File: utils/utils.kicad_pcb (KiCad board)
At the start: 2 copper layers, 34.8 x 69.8 mm, 22 parts, among them J6 EURORACK_CONN_16, Q1 2N3904, Q2 2N3904, Q3 2N3904, U1 TL074, U2 DG403

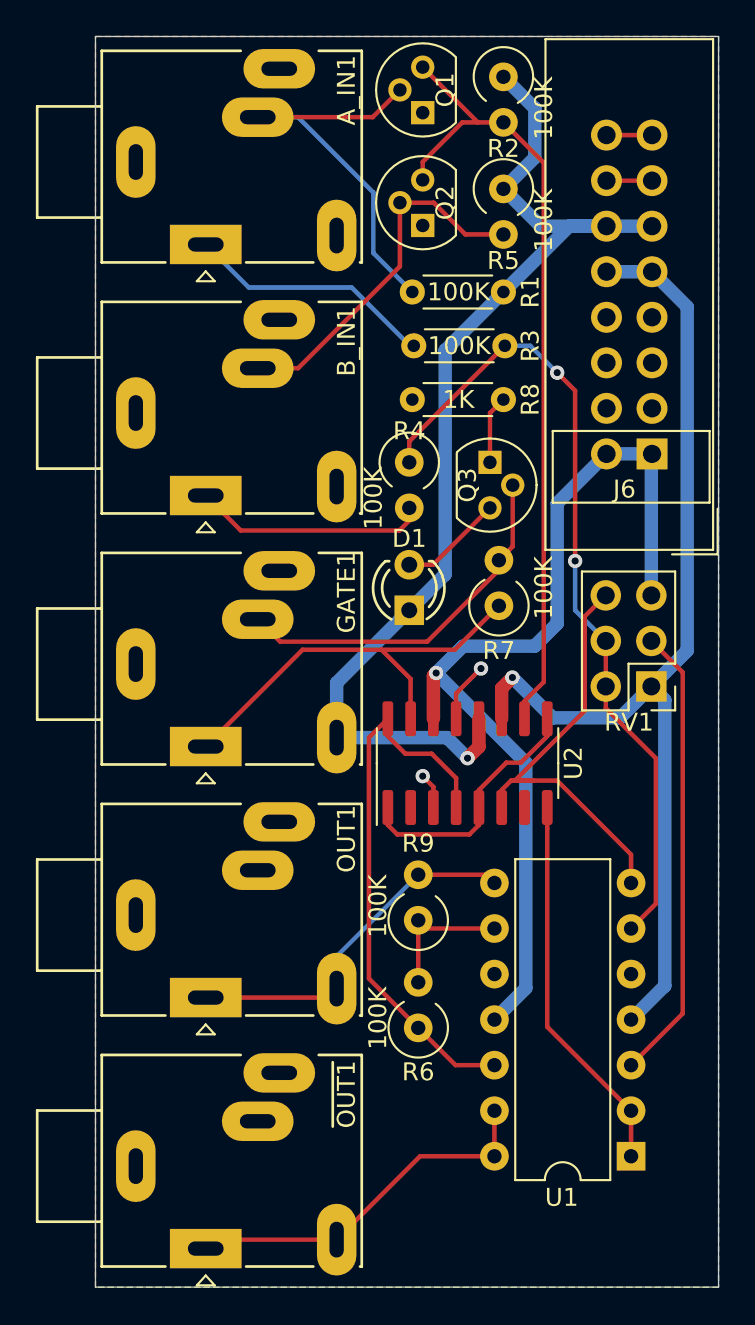
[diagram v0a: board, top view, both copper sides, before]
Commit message: cleanup
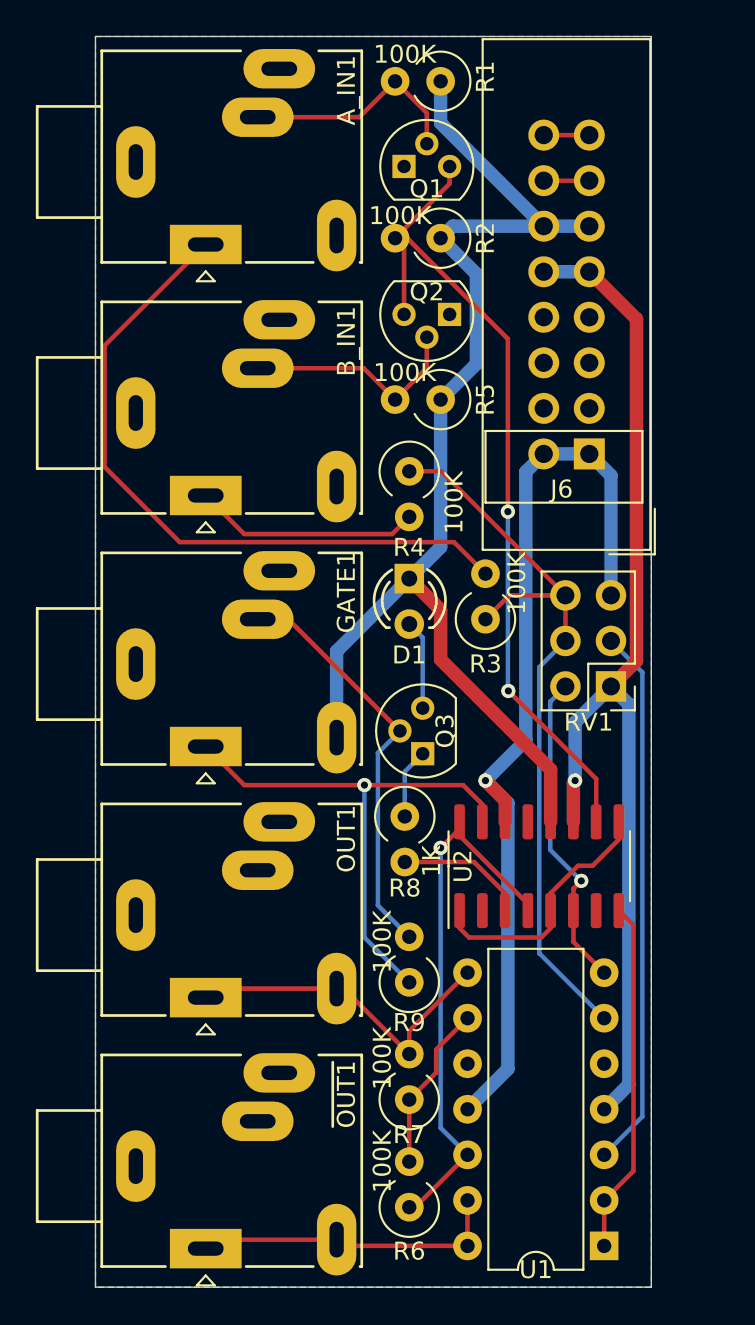
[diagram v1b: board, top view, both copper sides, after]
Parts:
- R1, R3, R8: footprint Resistor_THT:R_Axial_DIN0204_L3.6mm_D1.6mm_P5.08mm_Horizontal -> Resistor_THT:R_Axial_DIN0309_L9.0mm_D3.2mm_P2.54mm_Vertical
- moved R8 23.9 mm to (140.5, 86.5), turned to 270 degrees
- moved R7 21.6 mm to (140.8, 95.8)
- moved Q3 16.7 mm to (141.5, 83.0), turned to 90 degrees
- moved R3 15.3 mm to (145.0, 75.5), turned to 90 degrees
- moved R1 12.3 mm to (142.5, 45.5)
- moved R5 12.3 mm to (142.5, 63.2), turned to 180 degrees
- moved R6 10.0 mm to (140.8, 108.3)
- moved R9 10.0 mm to (140.8, 102.3)
- moved R2 9.66 mm to (142.5, 54.2), turned to 180 degrees
- moved U2 7.00 mm to (148.0, 89.3)
- moved U1 5.22 mm to (151.6, 110.5)
- moved Q2 5.18 mm to (143.0, 58.5), turned to 180 degrees
- moved J6 3.50 mm to (150.8, 66.3)
- moved Q1 3.18 mm to (140.5, 50.2), turned to 0 degrees
- moved RV1 2.25 mm to (152.0, 79.2)
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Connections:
- RV1 pad 4: Net-(R3-Pad1) -> Net-(RV1-Pad4)
- RV1 pad 6: Net-(RV1-Pad6) -> Net-(R3-Pad1)
- U1 pad 7: Net-(RV1-Pad6) -> Net-(RV1-Pad4)
- U2 pad 6: Net-(RV1-Pad6) -> Net-(RV1-Pad4)
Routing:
- net Net-(RV1-Pad6): track 25.6 -> 0.00 mm
- net AIN: track 13.7 -> 38.5 mm
- net Net-(RV1-Pad4): track 0.00 -> 17.9 mm, vias 0 -> 1
- net A_CONN: track 23.2 -> 12.7 mm
- net B_CONN: track 20.3 -> 12.6 mm
- net GATE: track 24.1 -> 29.8 mm, vias 0 -> 1
- net Net-(RV1-Pad2): track 25.6 -> 30.3 mm
- net ~OUT: track 21.9 -> 17.5 mm
- net Net-(R3-Pad1): track 46.1 -> 42.3 mm, vias 2 -> 0
- net +5V: track 64.3 -> 67.8 mm, vias 1 -> 0
- net GATE_CONN: track 20.7 -> 23.2 mm
- net GND: track 5.75 -> 7.67 mm, vias 2 -> 0
- net CONST: track 45.4 -> 47.3 mm, vias 0 -> 2
- net +12V: track 58.9 -> 60.7 mm
- net Net-(U1-Pad1): track 21.4 -> 19.7 mm
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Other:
- board size 34.8 x 69.8 mm -> 31 x 69.8 mm
- board text added: "TODO: verify switch direction"
